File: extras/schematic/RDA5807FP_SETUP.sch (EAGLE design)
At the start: 17 parts, among them Q1 32768k, U1 ESP32-DEVKITC-32D, X1 HD44780LCD-1602

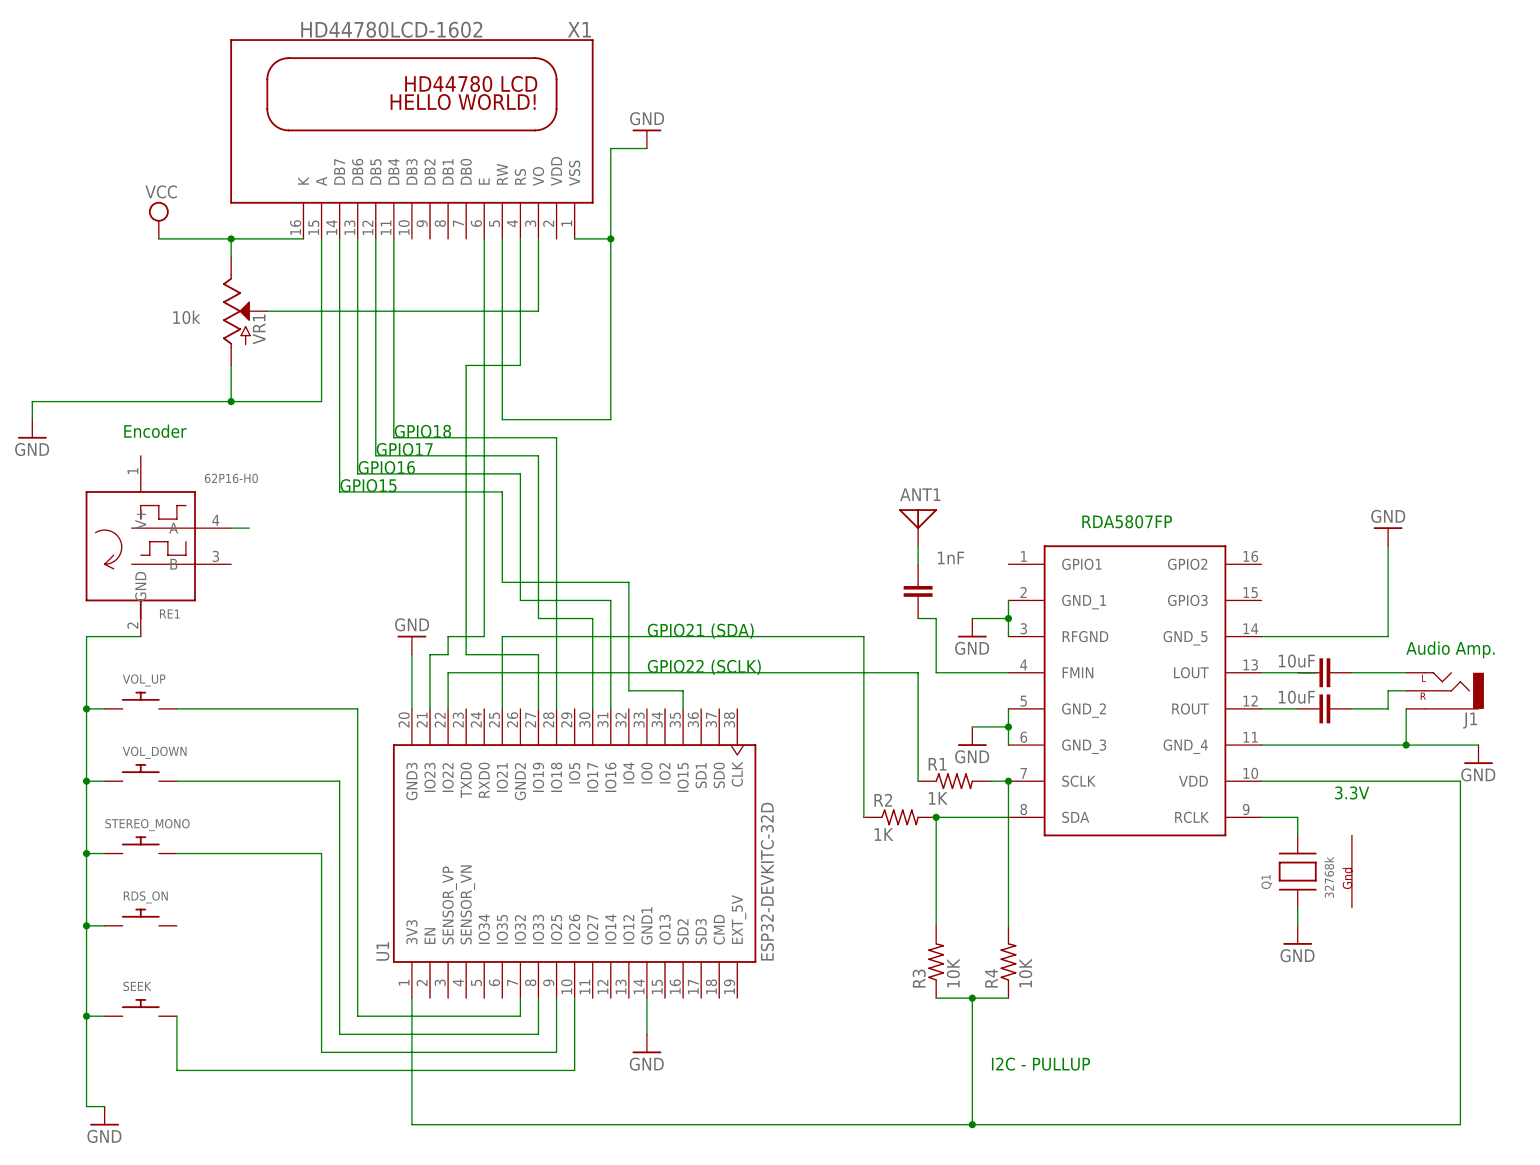
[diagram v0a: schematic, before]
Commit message: RDA5807 Arduino Library
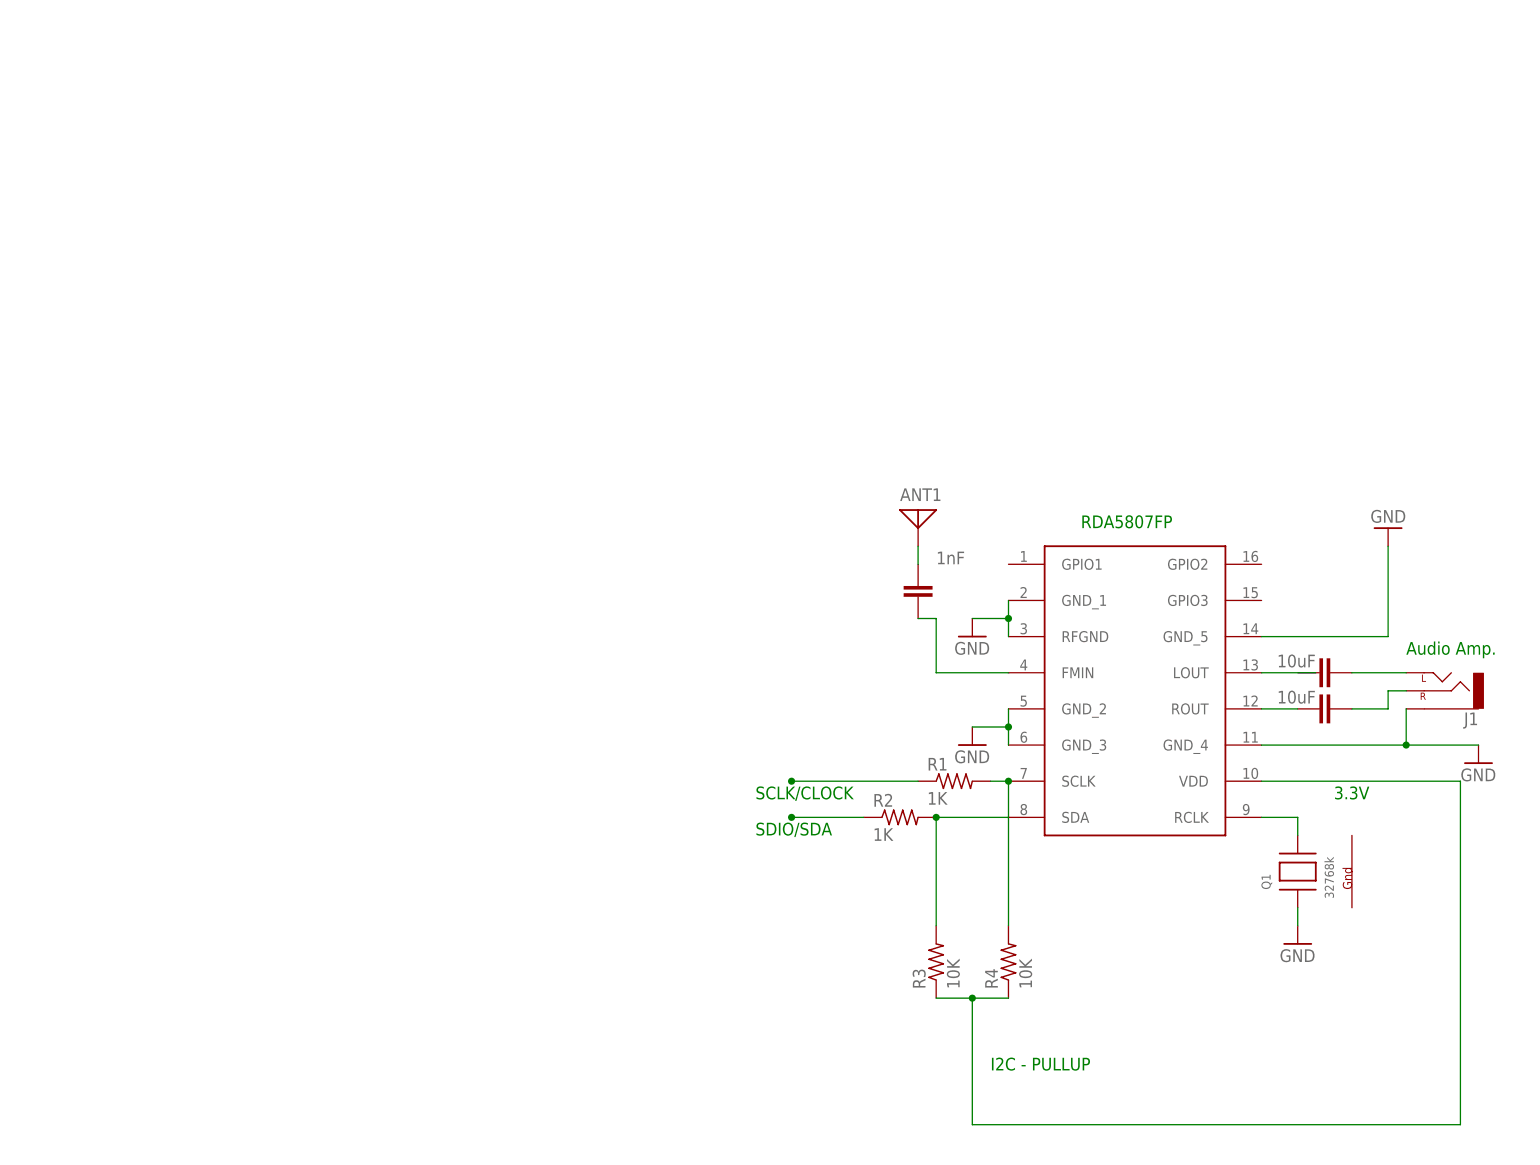
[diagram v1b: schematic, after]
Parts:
- removed RDS_ON, SEEK, STEREO_MONO, VOL_DOWN, VOL_UP: (no value), adafruit:SWITCH_PUSHBUTTONC&K_KSS
- removed RE1: 62P16-H0, rotary-encoder:62P16-H0
- removed U1: ESP32-DEVKITC-32D, ESP32-DEVKITC-32D:ESP32-DEVKITC-32D
- removed VR1: 10k, SparkFun-Resistors:POTENTIOMETER-PTH-9MM-1/20W-20%
- removed X1: HD44780LCD-1602, adafruit:HD44780LCD-1602
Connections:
- removed net N$10: STEREO_MONO.P$2, U1.IO25
- removed net N$14: VR1.S, X1.VO
- removed net N$15: U1.IO18, X1.DB4
- removed net N$16: RE1.A
- removed net N$17: U1.IO17, X1.DB5
- removed net N$18: U1.IO16, X1.DB6
- removed net N$19: U1.IO15, X1.DB7
- removed net N$20: U1.IO32, VOL_UP.P$2
- removed net N$21: SEEK.P$2, U1.IO26
- removed net N$22: U1.IO33, VOL_DOWN.P$2
- removed net N$23: U1.IO19, X1.RS
- removed net N$24: U1.IO23, X1.E
- removed net VCC: VR1.E, X1.K
- removed net VSS: X1.RW, X1.VSS
- net GND: no longer RDS_ON.P$1, RE1.GND, SEEK.P$1, STEREO_MONO.P$1, U1.GND1, U1.GND3, VOL_DOWN.P$1, VOL_UP.P$1, VR1.A, X1.A
- net N$4: now also R1.1; no longer R2.1, U1.IO21
- net N$5: now also R2.1; no longer R1.1, U1.IO22
- net N$6: no longer U1.3V3
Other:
- note added: "SCLK/CLOCK"
- note added: "SDIO/SDA"
- note removed: "Encoder"
- note removed: "GPIO15"
- note removed: "GPIO16"
- note removed: "GPIO17"
- note removed: "GPIO18"
- note removed: "GPIO21 (SDA)"
- note removed: "GPIO22 (SCLK)"
